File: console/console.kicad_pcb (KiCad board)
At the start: 2 copper layers, 15 parts

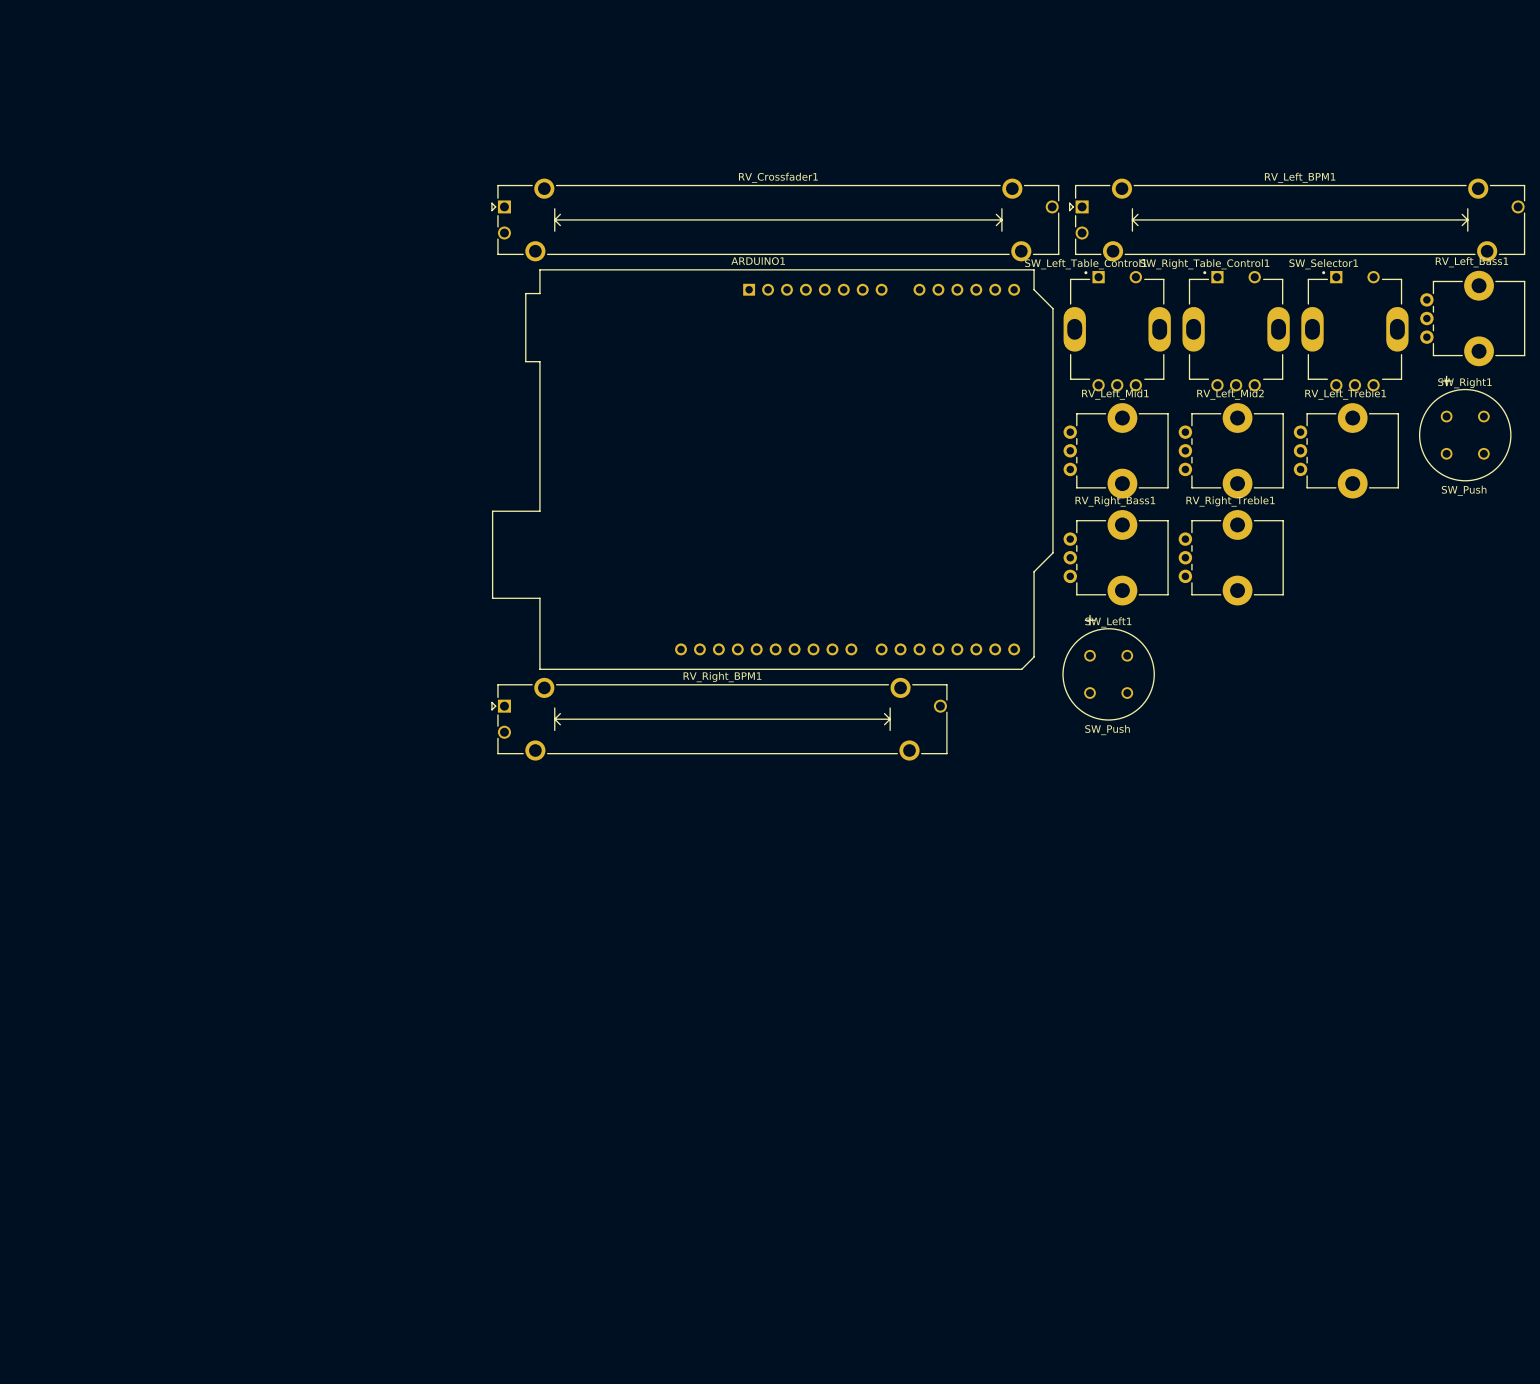
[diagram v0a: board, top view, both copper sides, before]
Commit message: PCB complete, not tested yet
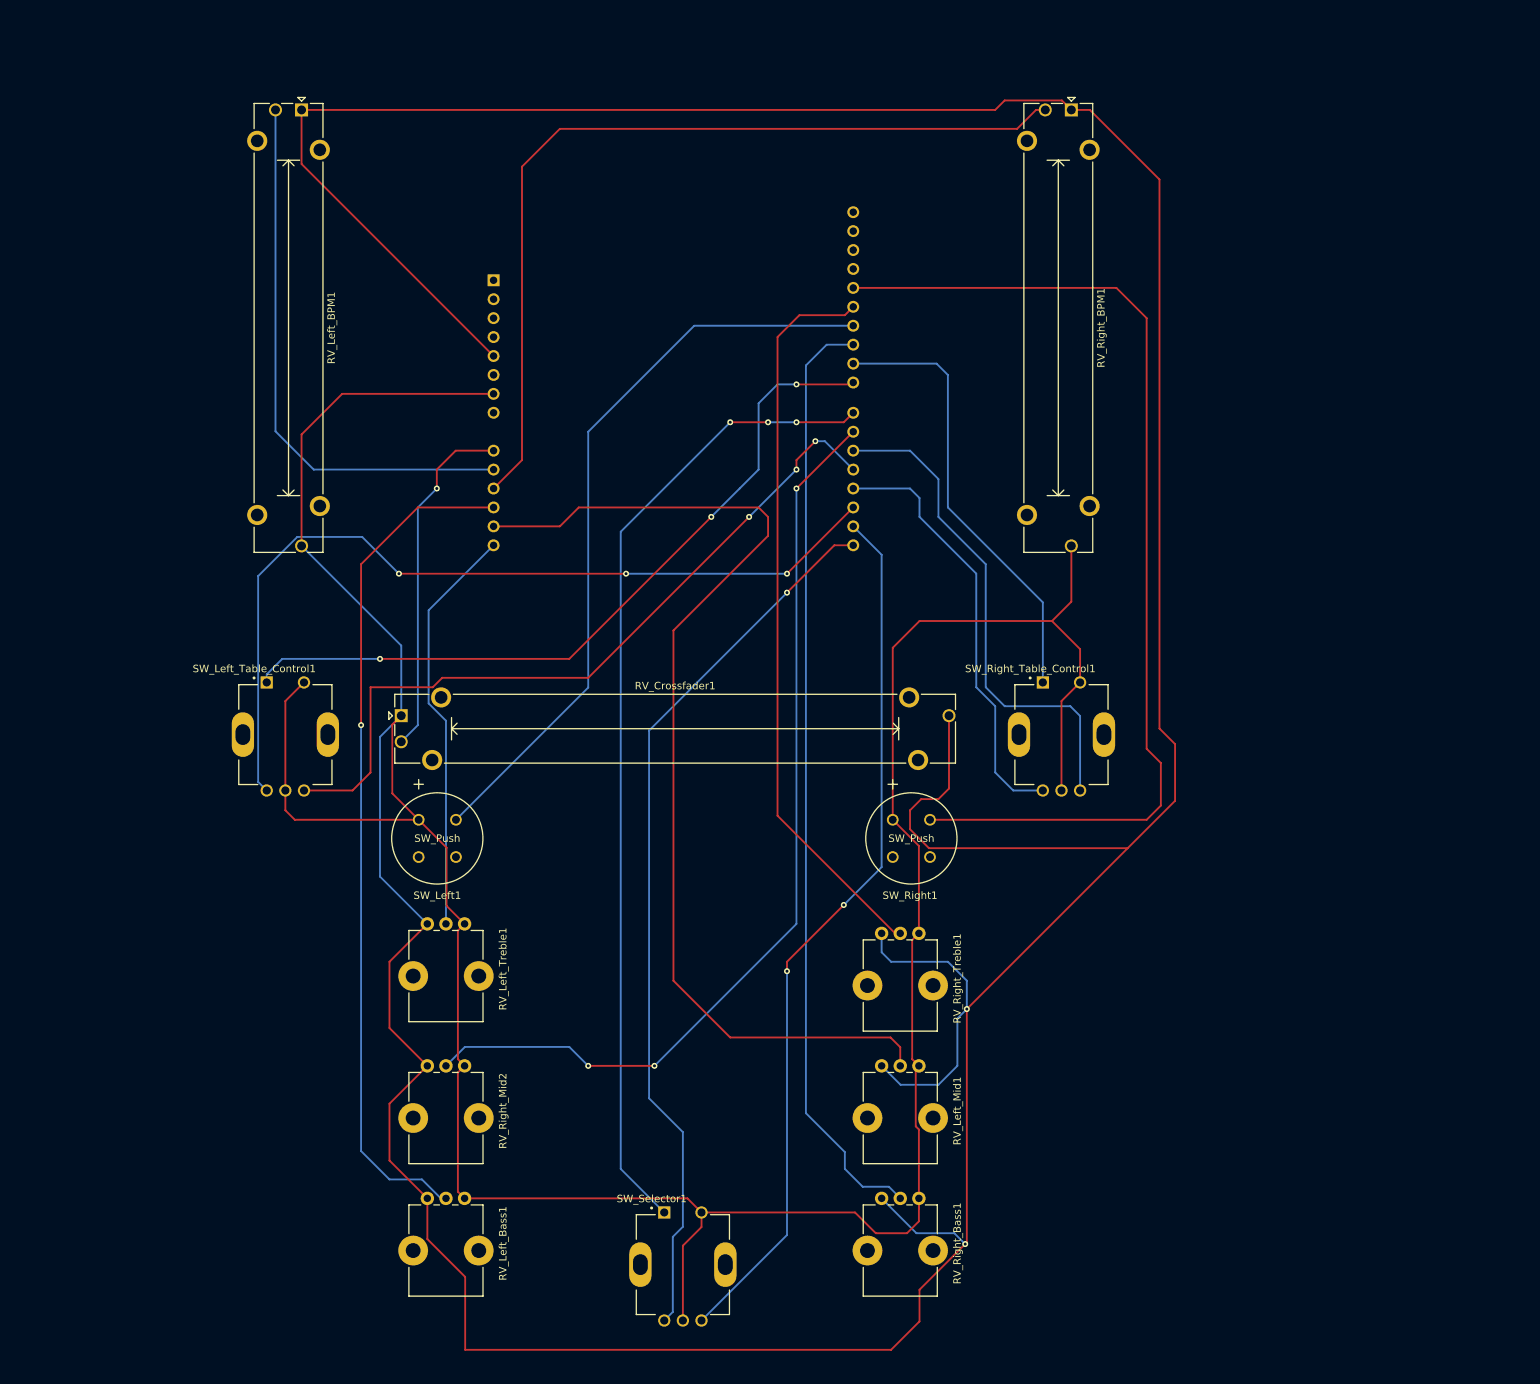
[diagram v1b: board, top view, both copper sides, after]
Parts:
- ARDUINO1: moved to B.Cu
- SW_Left1, SW_Right1: footprint footprints custom 1:D6R90F2LFS -> digikey-footprints:D6R90F2LFS
- SW_Left_Table_Control1, SW_Right_Table_Control1, SW_Selector1: footprint footprints custom 2:XDCR_PEC11R-4215F-S0024 -> digikey-footprints:XDCR_PEC11R-4215F-S0024
- moved RV_Left_Bass1 177.0 mm to (80.0, 171.4), turned to 270 degrees
- moved SW_Selector1 154.5 mm to (114.3, 180.3)
- moved RV_Left_Treble1 132.1 mm to (80.0, 134.6), turned to 270 degrees
- moved RV_Right_Mid2 129.4 mm to (80.0, 153.7), turned to 270 degrees
- moved SW_Left_Table_Control1 124.2 mm to (61.0, 109.2)
- moved RV_Right_BPM1 110.4 mm to (166.4, 25.4), turned to 270 degrees
- moved RV_Left_BPM1 105.5 mm to (63.1, 25.4), turned to 270 degrees
- moved SW_Left1 92.7 mm to (78.8, 120.7)
- moved SW_Right1 91.9 mm to (142.5, 120.7)
- moved RV_Right_Bass1 87.2 mm to (141.0, 171.4), turned to 270 degrees
- moved RV_Left_Mid1 83.9 mm to (141.0, 153.7), turned to 270 degrees
- moved RV_Crossfader1 69.7 mm to (76.5, 106.7)
- moved RV_Right_Treble1 62.9 mm to (141.0, 135.9), turned to 270 degrees
- moved SW_Right_Table_Control1 59.2 mm to (165.1, 109.2)
- moved ARDUINO1 34.3 mm to (88.9, 48.3), turned to 270 degrees
- renumbered RV_Left_Mid2 to RV_Right_Mid2
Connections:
- RV_Crossfader1 pad 1: Net-(ARDUINO1-Pad5) -> Net-(ARDUINO1-Pad7)
- RV_Crossfader1 pad 2: Net-(RV_Crossfader1-Pad2) -> Net-(ARDUINO1-Pad9)
- RV_Crossfader1 pad 3: Net-(ARDUINO1-Pad7) -> Net-(ARDUINO1-Pad5)
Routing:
- net Net-(ARDUINO1-Pad5): track 0.00 -> 597.2 mm, vias 0 -> 2
- net Net-(ARDUINO1-Pad7): track 0.00 -> 397.7 mm
- net Net-(ARDUINO1-Pad13): track 0.00 -> 142.5 mm
- net Net-(ARDUINO1-Pad28): track 0.00 -> 139.0 mm
- net Net-(ARDUINO1-Pad22): track 0.00 -> 131.6 mm, vias 0 -> 3
- net Net-(ARDUINO1-Pad25): track 0.00 -> 126.6 mm
- net Net-(ARDUINO1-Pad21): track 0.00 -> 126.2 mm, vias 0 -> 3
- net Net-(ARDUINO1-Pad15): track 0.00 -> 119.8 mm, vias 0 -> 1
- net Net-(ARDUINO1-Pad16): track 0.00 -> 118.1 mm, vias 0 -> 2
- net Net-(ARDUINO1-Pad11): track 0.00 -> 118.1 mm
- net Net-(ARDUINO1-Pad17): track 0.00 -> 117.0 mm, vias 0 -> 3
- net Net-(ARDUINO1-Pad12): track 0.00 -> 113.7 mm, vias 0 -> 1
- net Net-(ARDUINO1-Pad19): track 0.00 -> 102.1 mm, vias 0 -> 3
- net Net-(ARDUINO1-Pad23): track 0.00 -> 101.2 mm, vias 0 -> 3
- net Net-(ARDUINO1-Pad26): track 0.00 -> 100.9 mm
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
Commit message: added edges
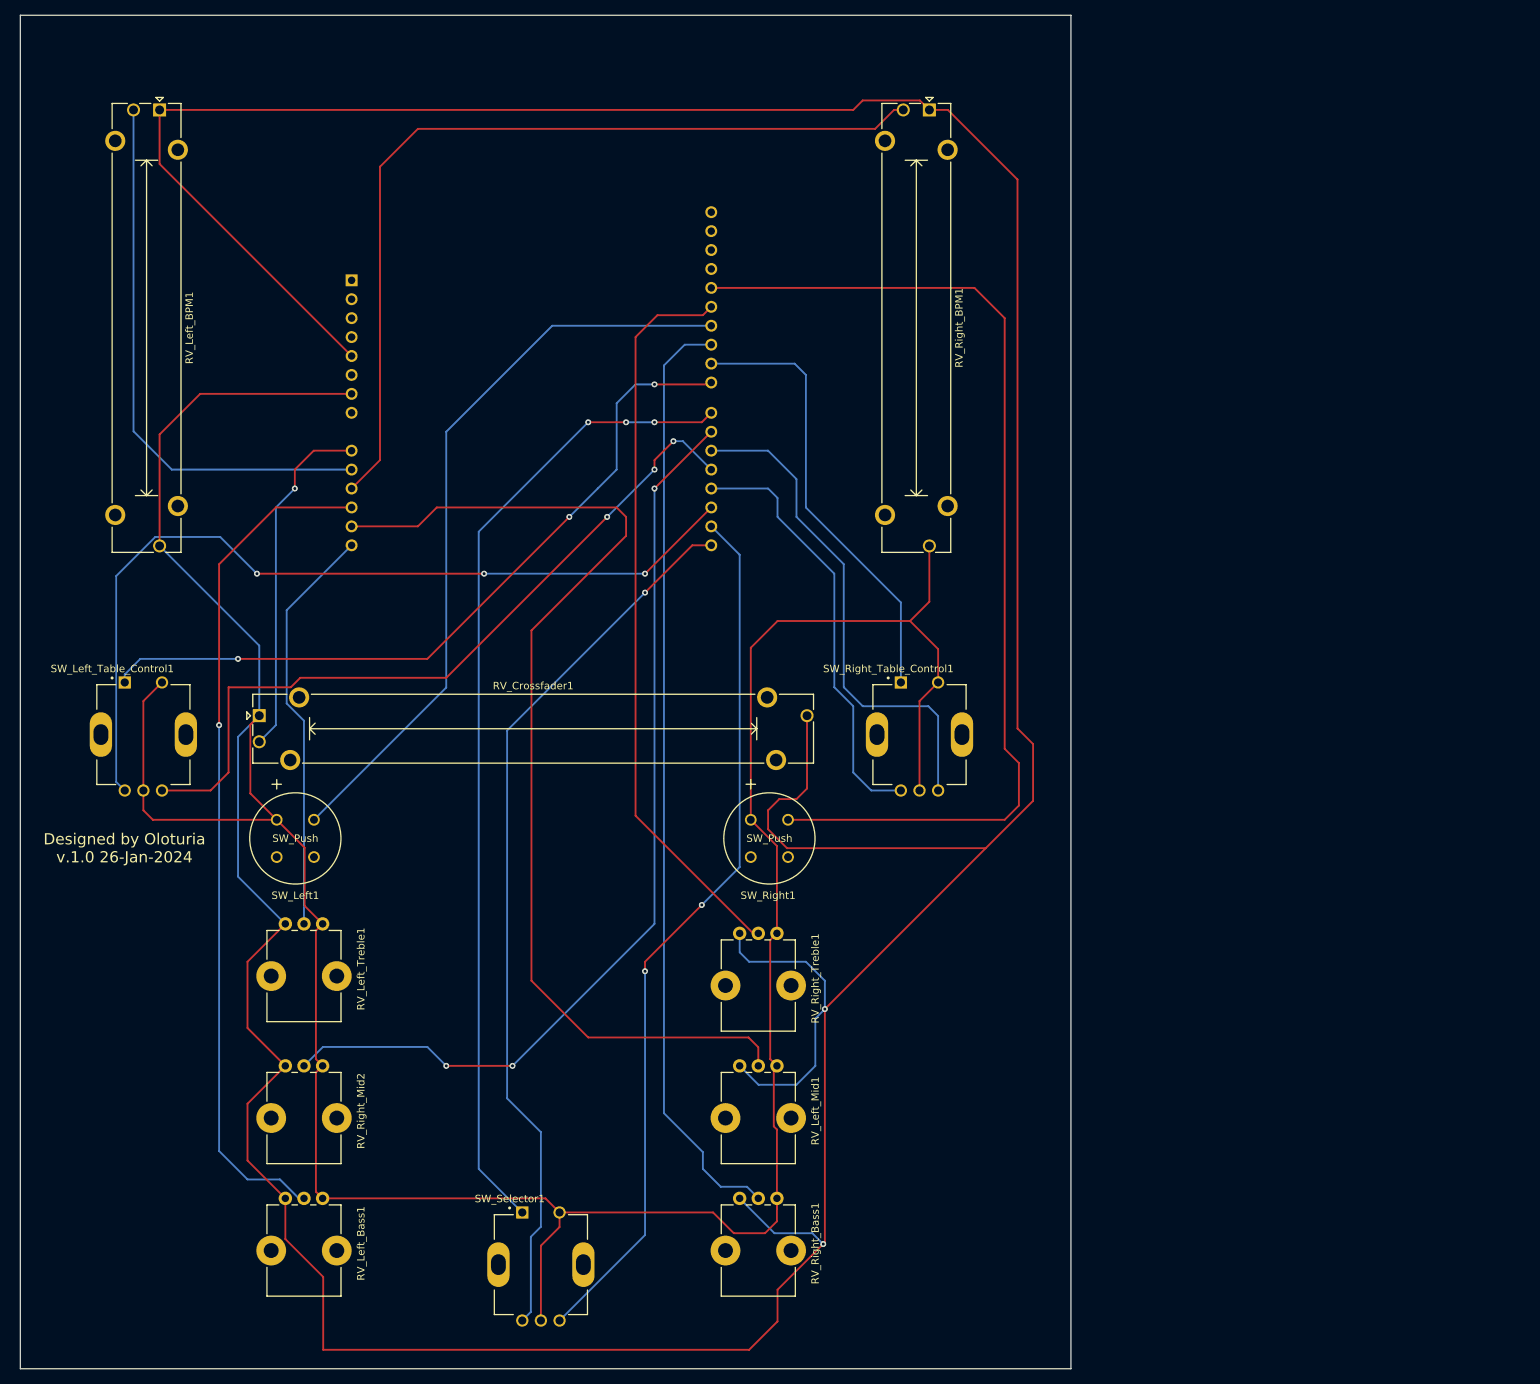
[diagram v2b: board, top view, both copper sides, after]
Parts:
- moved ARDUINO1 19.1 mm to (69.8, 48.3)
- moved RV_Right_BPM1 19.1 mm to (147.4, 25.4)
- moved RV_Crossfader1 19.1 mm to (57.5, 106.7)
- moved RV_Left_Bass1 19.1 mm to (61.0, 171.4)
- moved RV_Left_Treble1 19.1 mm to (61.0, 134.6)
- moved RV_Right_Mid2 19.1 mm to (61.0, 153.7)
- moved SW_Left_Table_Control1 19.1 mm to (41.9, 109.2)
- moved RV_Left_BPM1 19.0 mm to (44.1, 25.4)
- moved RV_Left_Mid1 19.0 mm to (121.9, 153.7)
- moved RV_Right_Bass1 19.0 mm to (121.9, 171.4)
- moved RV_Right_Treble1 19.0 mm to (121.9, 135.9)
- moved SW_Left1 19.0 mm to (59.8, 120.7)
- moved SW_Right1 19.0 mm to (123.4, 120.7)
- moved SW_Selector1 19.0 mm to (95.2, 180.3)
- moved SW_Right_Table_Control1 19.0 mm to (146.1, 109.2)
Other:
- board outline added: 141 x 181.6 mm
- board text added: "Designed by Oloturia v.1.0 26-Jan-2024"
